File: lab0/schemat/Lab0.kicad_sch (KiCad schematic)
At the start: 5 parts

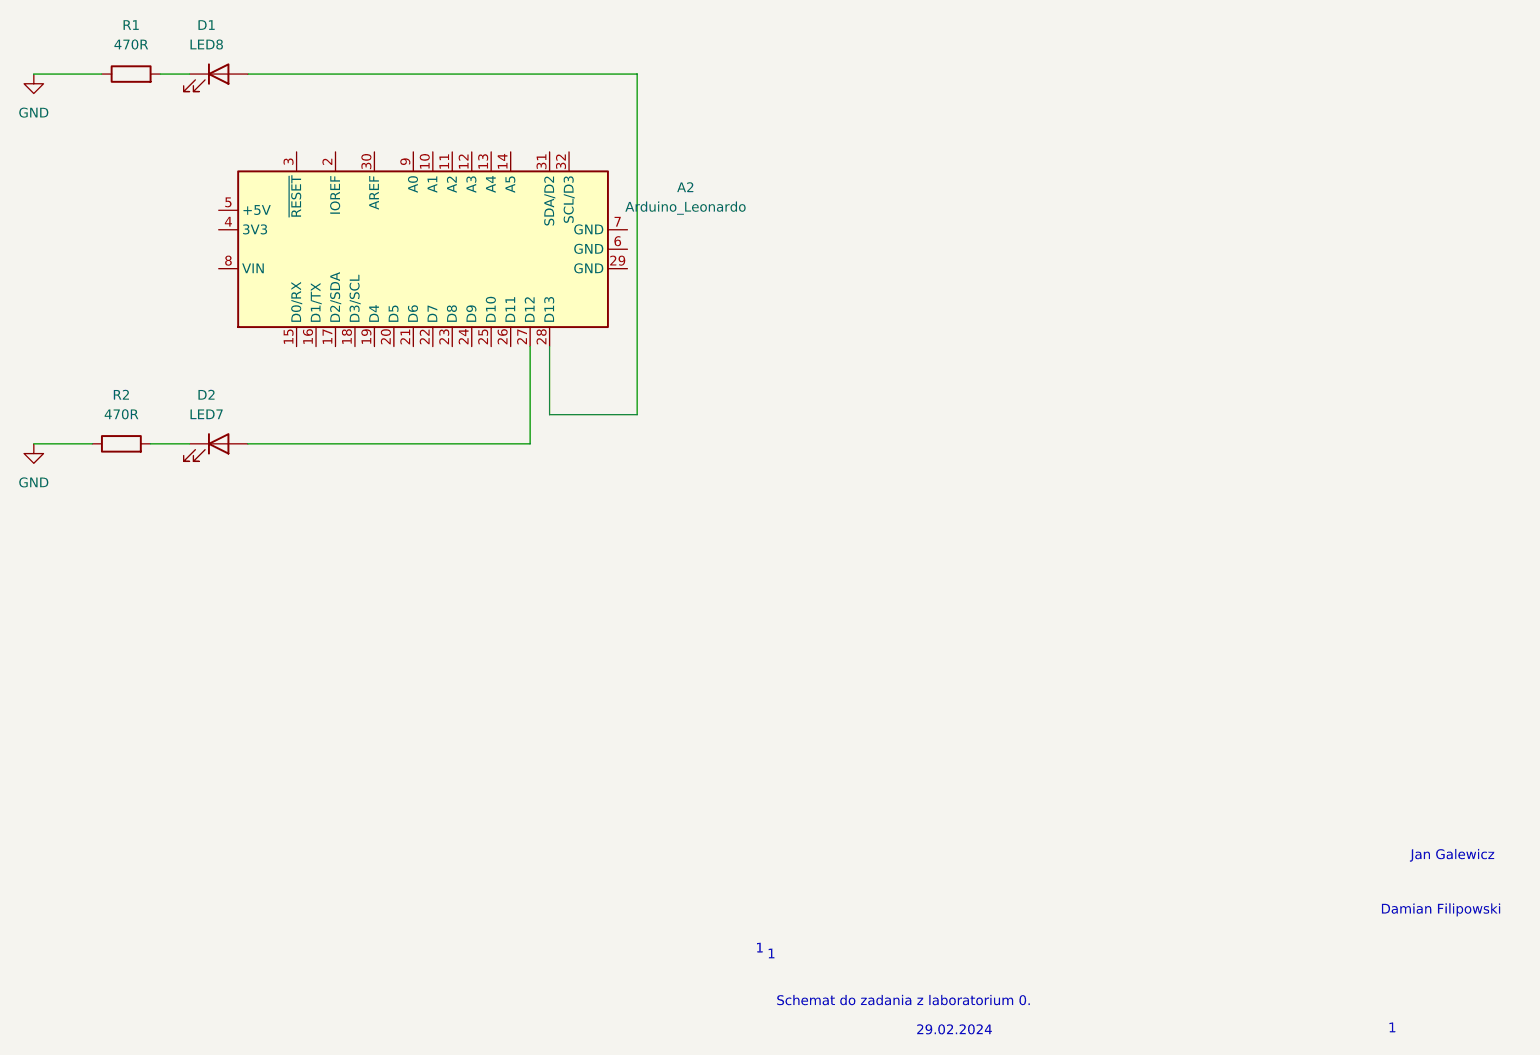
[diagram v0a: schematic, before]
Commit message: Fix scheme
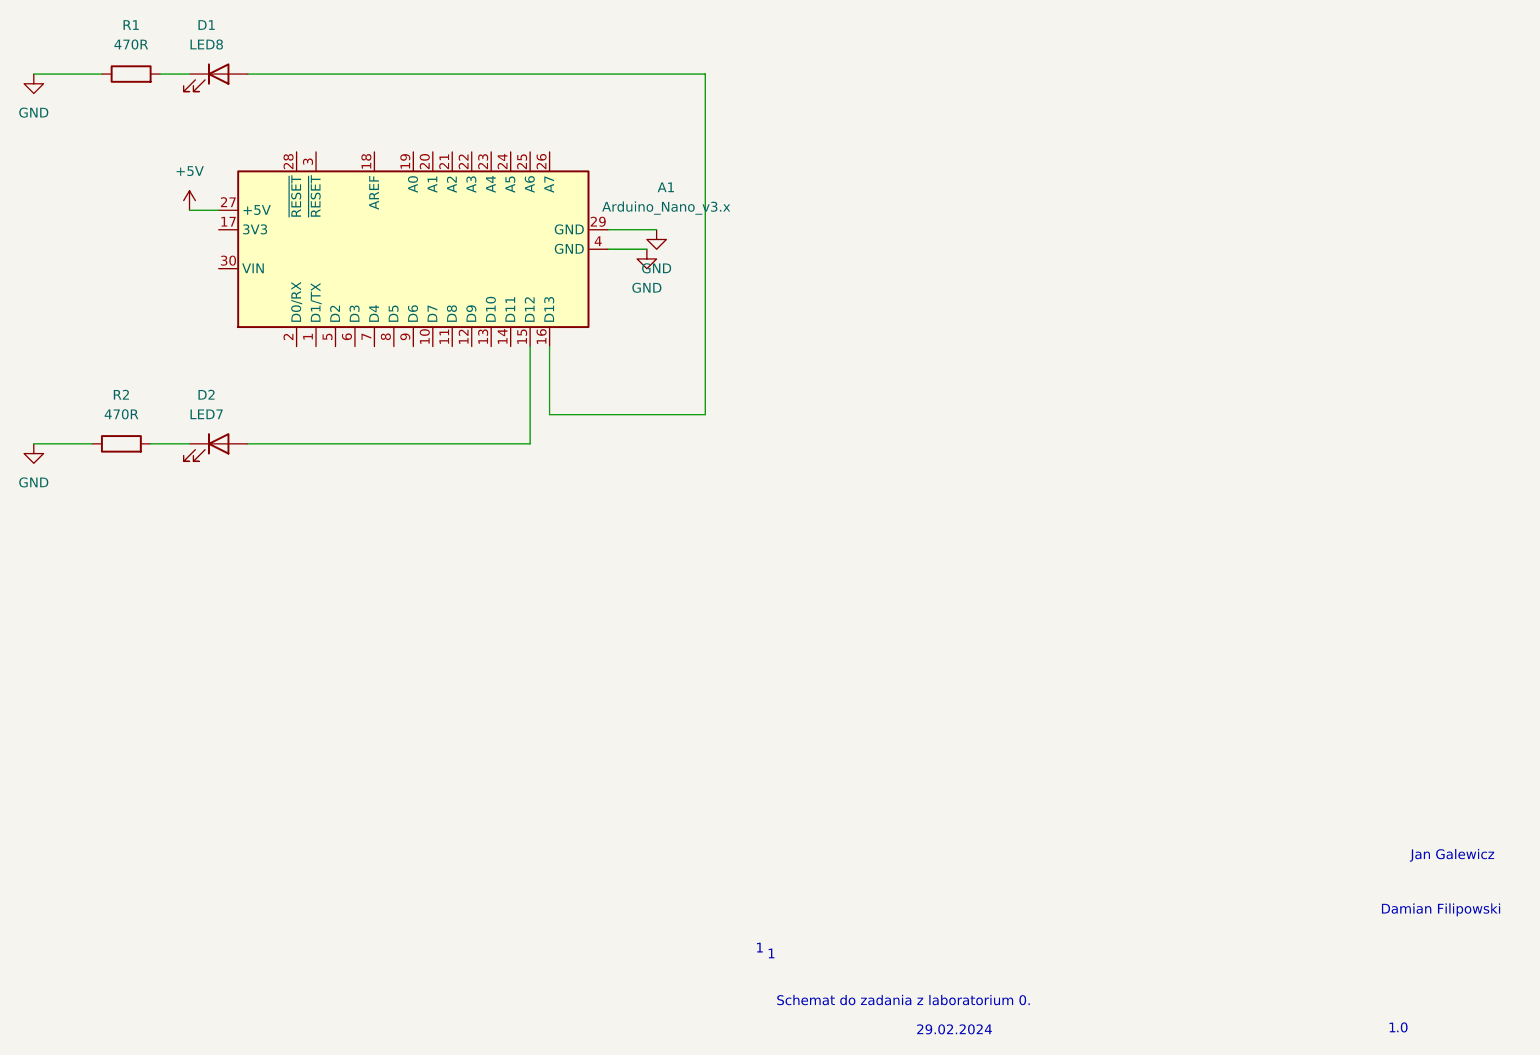
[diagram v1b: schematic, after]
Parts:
- removed A2: Arduino_Leonardo, Module:Arduino_UNO_R3, symbol MCU_Module:Arduino_Leonardo
- added A1: Arduino_Nano_v3.x, Module:Arduino_Nano, symbol MCU_Module:Arduino_Nano_v3.x
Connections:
- net GND: now also A1.29 (GND), A1.4 (GND)
- net at D1.2 (A): now also A1.16 (D13)
- net at D2.2 (A): now also A1.15 (D12)
- new net +5V: A1.27 (+5V)
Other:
- note added: ".0"
